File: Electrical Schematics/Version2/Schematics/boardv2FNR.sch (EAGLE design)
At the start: 36 parts, among them IC1 MCP41HVX1ST, K1 G5V-2, Q1 IRLML2060TRPBFBSS123LT1G, Q2 IRLML2060TRPBFBSS123LT1G, Q3 IRLML2060TRPBFBSS123LT1G, Q4 IRLML2060TRPBFBSS123LT1G, Q5 IRLML2060TRPBFBSS123LT1G, Q6 IRLML2060TRPBFBSS123LT1G

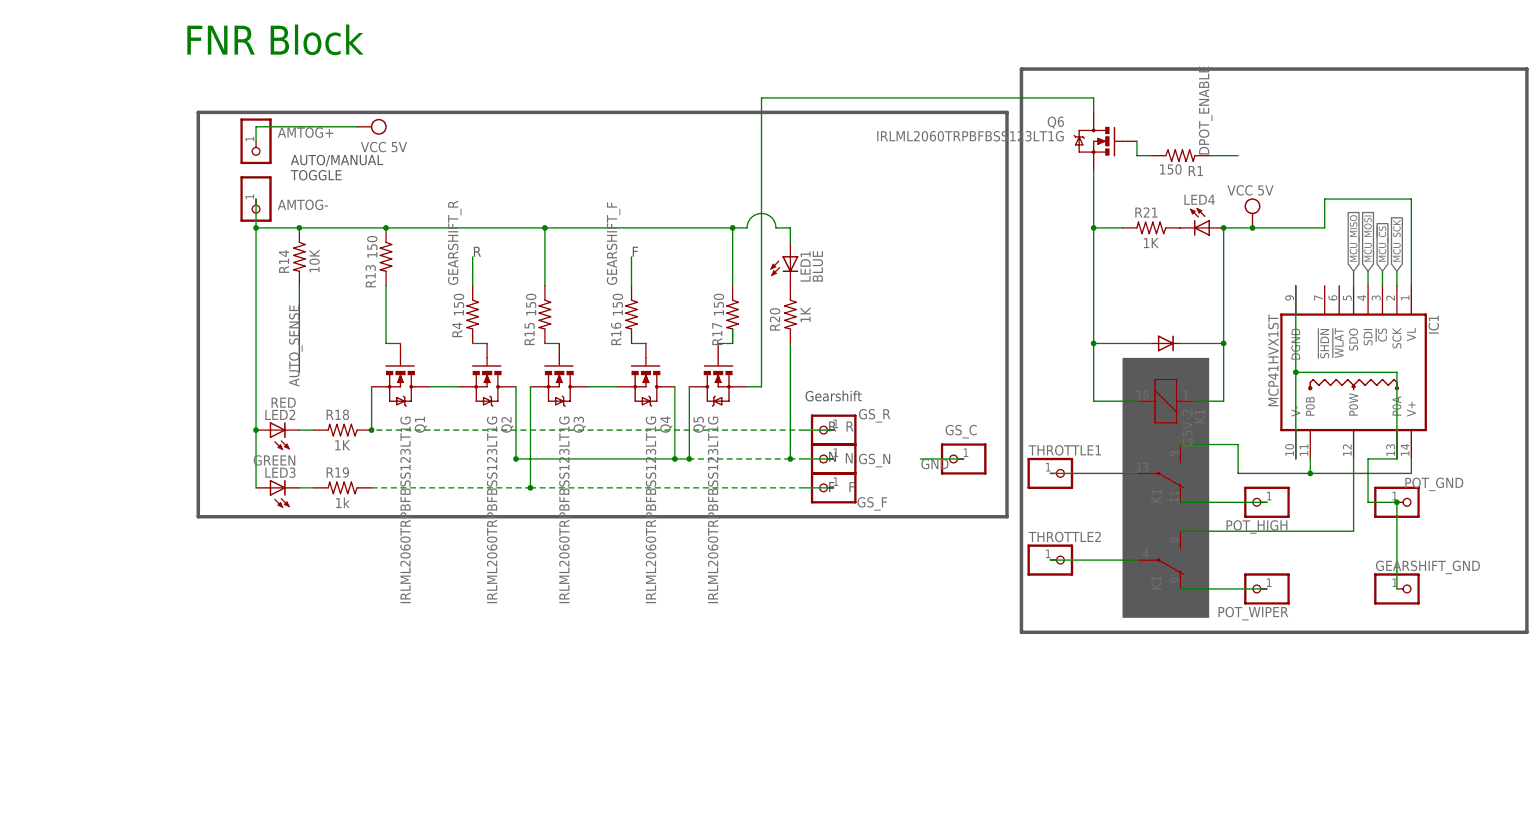
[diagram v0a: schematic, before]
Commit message: updated fnr
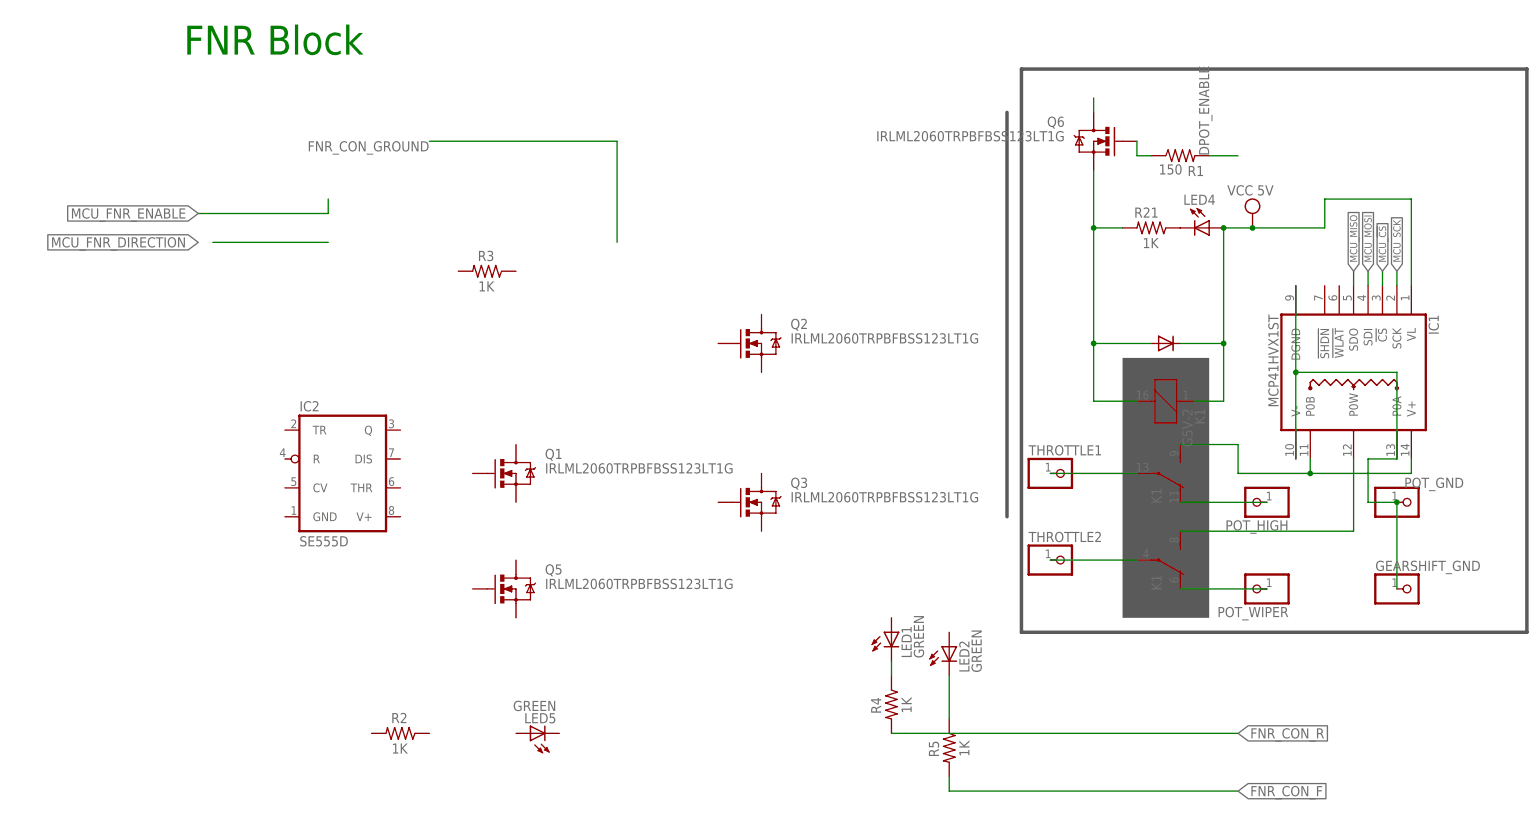
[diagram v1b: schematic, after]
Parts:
- removed AMTOG+, AMTOG-: (no value), adafruit:PINHD-1X1
- removed GS_C, GS_N: N, adafruit:PINHD-1X1
- removed GS_F: F, adafruit:PINHD-1X1
- removed GS_R: R, adafruit:PINHD-1X1
- removed LED3: GREEN, adafruit:LED3MM
- removed Q4: IRLML2060TRPBFBSS123LT1G, SparkFun-DiscreteSemi:IRLML2060TRPBFBSS123LT1G
- removed R13, R15, R16, R17: 150, rcl:R-US_0204/5
- removed R14: 10K, rcl:R-US_0204/5
- removed R18, R20: 1K, rcl:R-US_0204/5
- removed R19: 1k, rcl:R-US_0204/5
- added IC2: SE555D, linear:SE555D
- added LED5: GREEN, adafruit:LED3MM
- added R2, R3, R5: 1K, rcl:R-US_0204/5
- LED1: value BLUE -> GREEN
- LED2: value RED -> GREEN
- R4: value 150 -> 1K
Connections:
- removed net AM_TOGGLE-: AMTOG-.1, LED1.A, LED2.A, LED3.A, R13.1, R14.1, R15.1, R17.1
- removed net AUTO_SENSE: R14.2
- removed net FGND: GS_F.1, Q3.S, R19.1
- removed net GEARSHIFT_F: R16.1
- removed net GEARSHIFT_R: R4.1
- removed net N: GS_N.1, Q2.D, Q4.D, Q5.D, R20.2
- removed net N$13: LED2.C, R18.2
- removed net N$14: LED3.C, R19.2
- removed net N$18: Q1.G, R13.2
- removed net N$22: Q3.D, Q4.S
- removed net N$23: Q5.G, R17.2
- removed net N$5: Q1.D, Q2.S
- removed net N$6: Q4.G, R16.2
- removed net N$8: LED1.C, R20.1
- removed net RGND: GS_R.1, Q1.S, R18.1
- new net FNR_CON_F: R5.2
- new net FNR_CON_R: R4.2
- net +5V: no longer AMTOG+.1
- net GND: no longer GS_C.1
- net N$1: no longer Q5.S
- net N$3: now also LED1.C, R4.1; no longer Q2.G, R4.2
- net N$4: now also LED2.C, R5.1; no longer Q3.G, R15.2
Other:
- note removed: "AUTO/MANUAL TOGGLE"
- note removed: "F"
- note removed: "Gearshift"
- note removed: "R"
- note removed: "R N F"
- moved on the sheet: LED1, LED2, Q1, Q2, Q3, Q5, R4
